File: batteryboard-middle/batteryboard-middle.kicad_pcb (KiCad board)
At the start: 2 copper layers, 46.8 x 46.8 mm, 9 parts, among them J1 FLE-107-01-G-DV-A, J2 Conn_01x02, J3 Conn_01x02, J4 FTS-107-01-L-DV-A

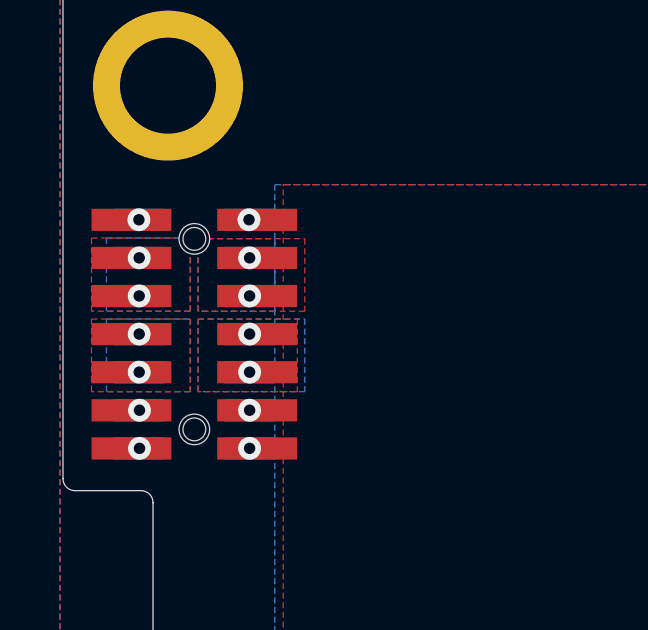
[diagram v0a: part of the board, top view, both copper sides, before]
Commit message: B2/01 Updates
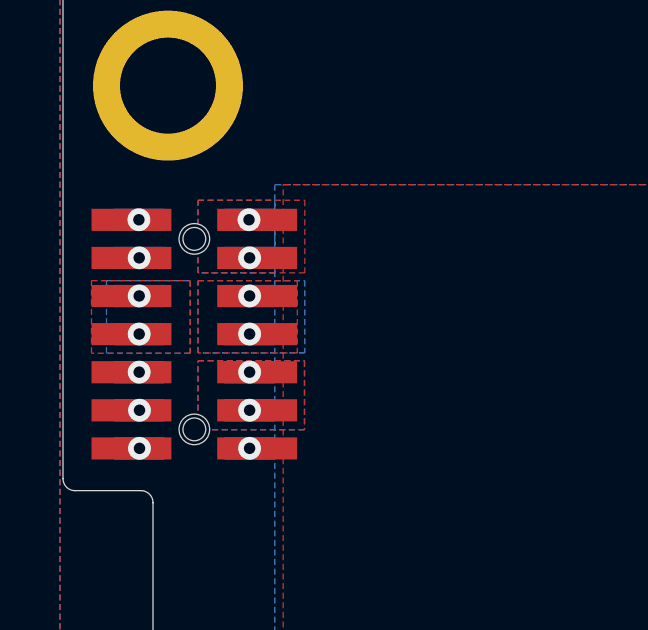
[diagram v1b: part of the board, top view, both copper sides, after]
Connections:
- J1 pad 10: BATT_N_SW -> BATT_P
- J1 pad 11: SCL1 -> SDA1
- J1 pad 12: COIL5_P -> BATT_P
- J1 pad 13: SDA1 -> COIL5_P
- J1 pad 2: GND -> BATT_N_SW
- J1 pad 3: +3V3 -> GND
- J1 pad 4: BATT_P_SW -> BATT_N_SW
- J1 pad 7: BATT_P -> +3V3
- J1 pad 8: BATT_N_SW -> BATT_P_SW
- J1 pad 9: BATT_P -> SCL1
- J4 pad 10: BATT_N_SW -> BATT_P
- J4 pad 11: SCL1 -> SDA1
- J4 pad 12: COIL5_P -> BATT_P
- J4 pad 13: SDA1 -> COIL5_P
- J4 pad 2: GND -> BATT_N_SW
- J4 pad 3: +3V3 -> GND
- J4 pad 4: BATT_P_SW -> BATT_N_SW
- J4 pad 7: BATT_P -> +3V3
- J4 pad 8: BATT_N_SW -> BATT_P_SW
- J4 pad 9: BATT_P -> SCL1
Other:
- board text added: "09-OCT-22"
- board text removed: "06-SEP-22"
